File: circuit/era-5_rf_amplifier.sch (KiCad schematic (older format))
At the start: 9 parts, among them J1 CONN_01X04, J2 CONN_01X04, U1 ERA-5+

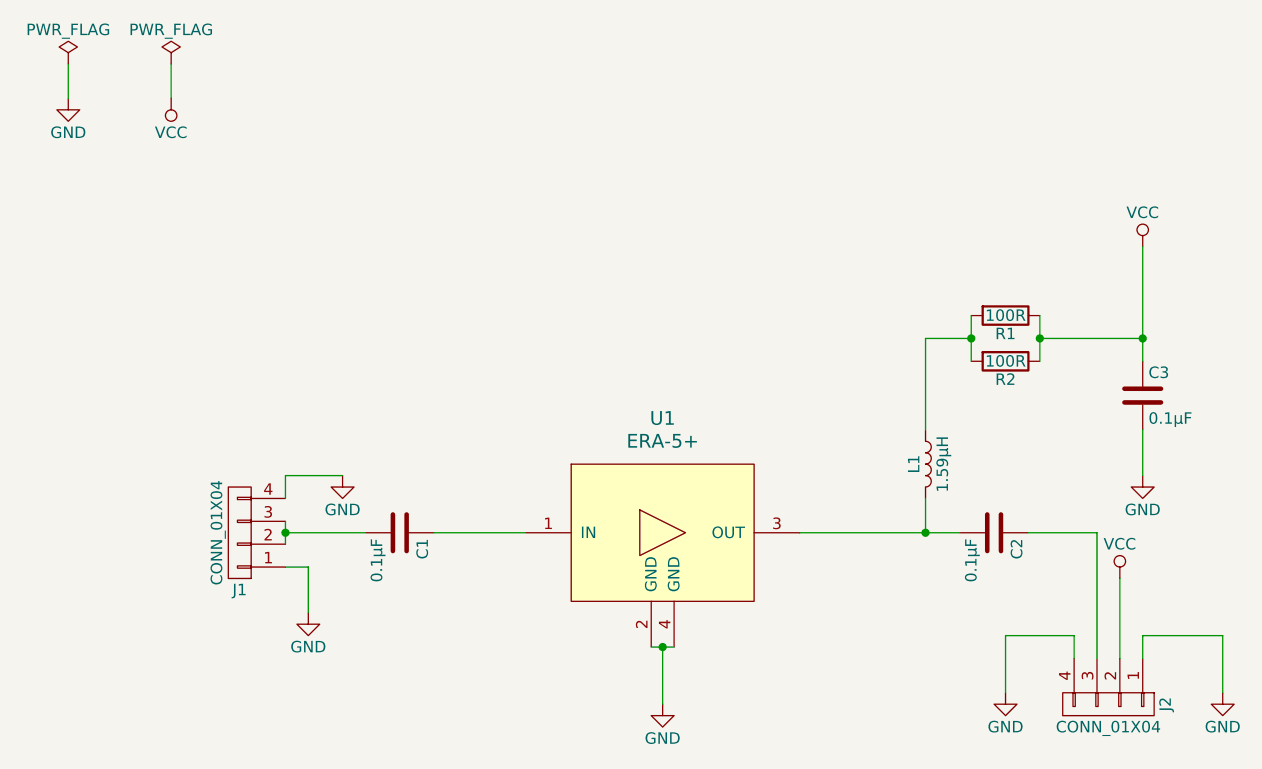
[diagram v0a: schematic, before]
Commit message: rearranged schematics
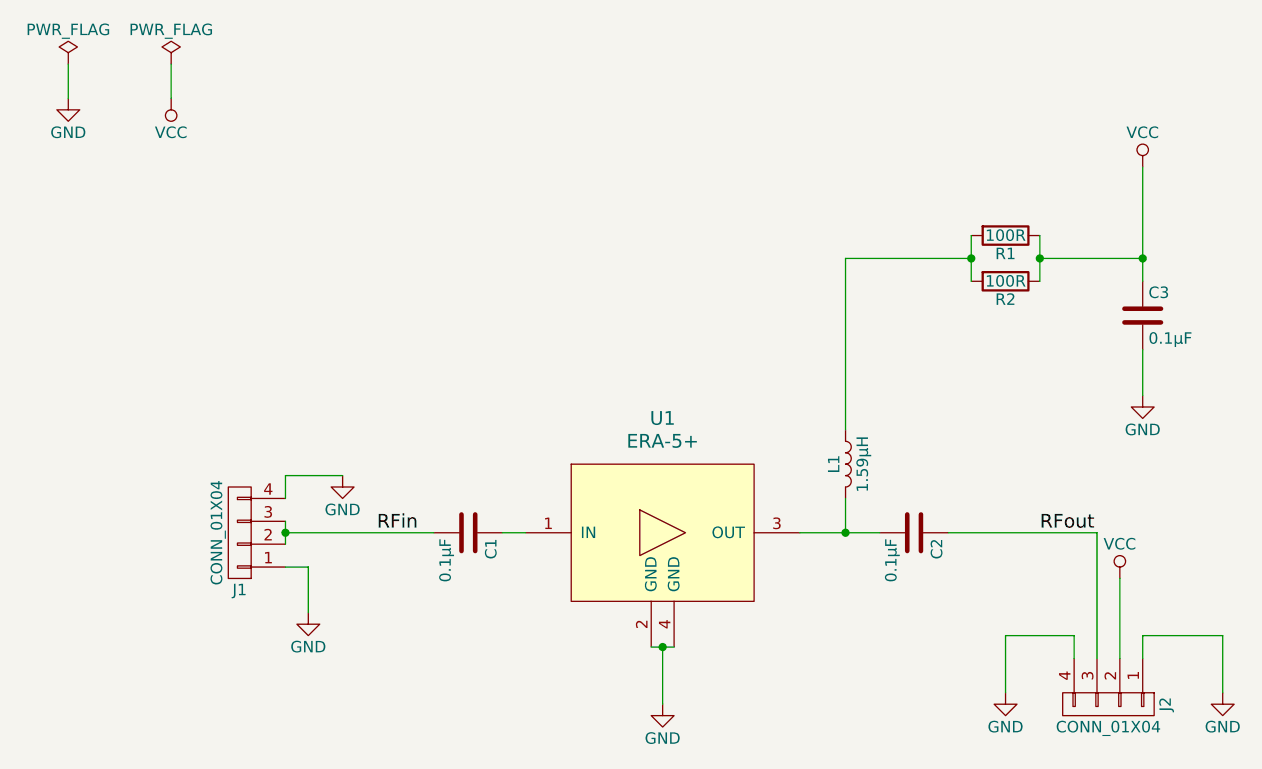
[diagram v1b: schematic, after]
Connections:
- net RFin: now reaches C1.2, J1.2 (P2), J1.3 (P3)
- net RFout: now reaches C2.1, J2.3 (P3)
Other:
- moved on the sheet: C1, C2, C3, L1, R1, R2
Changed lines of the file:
@@
 L C C1
 U 1 1 5931B134
-P 2550 2800
-F 0 "C1" H 2575 2900 50  0000 L CNN
-F 1 "0.1µF" H 2575 2700 50  0000 L CNN
-F 2 "" H 2588 2650 50  0001 C CNN
-F 3 "" H 2550 2800 50  0001 C CNN
-	1    2550 2800
+P 2850 2800
+F 0 "C1" H 2875 2900 50  0000 L CNN
+F 1 "0.1µF" H 2875 2700 50  0000 L CNN
+F 2 "" H 2888 2650 50  0001 C CNN
+F 3 "" H 2850 2800 50  0001 C CNN
+	1    2850 2800
 	0    1    1    0
 $EndComp
@@
 L C C2
 U 1 1 5931B1E4
-P 5150 2800
-F 0 "C2" H 5175 2900 50  0000 L CNN
-F 1 "0.1µF" H 5175 2700 50  0000 L CNN
-F 2 "" H 5188 2650 50  0001 C CNN
-F 3 "" H 5150 2800 50  0001 C CNN
-	1    5150 2800
+P 4800 2800
+F 0 "C2" H 4825 2900 50  0000 L CNN
+F 1 "0.1µF" H 4825 2700 50  0000 L CNN
+F 2 "" H 4838 2650 50  0001 C CNN
+F 3 "" H 4800 2800 50  0001 C CNN
+	1    4800 2800
 	0    1    1    0
 $EndComp
@@
 L L L1
 U 1 1 5931B2E5
-P 4850 2500
-F 0 "L1" V 4800 2500 50  0000 C CNN
-F 1 "1.59µH" V 4925 2500 50  0000 C CNN
-F 2 "" H 4850 2500 50  0001 C CNN
-F 3 "" H 4850 2500 50  0001 C CNN
-	1    4850 2500
+P 4500 2500
+F 0 "L1" V 4450 2500 50  0000 C CNN
+F 1 "1.59µH" V 4575 2500 50  0000 C CNN
+F 2 "" H 4500 2500 50  0001 C CNN
+F 3 "" H 4500 2500 50  0001 C CNN
+	1    4500 2500
 	1    0    0    -1
 $EndComp
@@
 L R R2
 U 1 1 5931B3DD
-P 5200 2050
-F 0 "R2" V 5280 2050 50  0000 C CNN
-F 1 "100R" V 5200 2050 50  0000 C CNN
-F 2 "" V 5130 2050 50  0001 C CNN
-F 3 "" H 5200 2050 50  0001 C CNN
-	1    5200 2050
+P 5200 1700
+F 0 "R2" V 5280 1700 50  0000 C CNN
+F 1 "100R" V 5200 1700 50  0000 C CNN
+F 2 "" V 5130 1700 50  0001 C CNN
+F 3 "" H 5200 1700 50  0001 C CNN
+	1    5200 1700
 	0    1    1    0
 $EndComp
@@
 L R R1
 U 1 1 5931B444
-P 5200 1850
-F 0 "R1" V 5280 1850 50  0000 C CNN
-F 1 "100R" V 5200 1850 50  0000 C CNN
-F 2 "" V 5130 1850 50  0001 C CNN
-F 3 "" H 5200 1850 50  0001 C CNN
-	1    5200 1850
+P 5200 1500
+F 0 "R1" V 5280 1500 50  0000 C CNN
+F 1 "100R" V 5200 1500 50  0000 C CNN
+F 2 "" V 5130 1500 50  0001 C CNN
+F 3 "" H 5200 1500 50  0001 C CNN
+	1    5200 1500
 	0    1    1    0
 $EndComp
@@
 L C C3
 U 1 1 5931B556
+P 5800 1850
+F 0 "C3" H 5825 1950 50  0000 L CNN
+F 1 "0.1µF" H 5825 1750 50  0000 L CNN
+F 2 "" H 5838 1700 50  0001 C CNN
+F 3 "" H 5800 1850 50  0001 C CNN
+	1    5800 1850
+	1    0    0    -1
+$EndComp
+$Comp
+L GND #PWR01
+U 1 1 5931B719
 P 5800 2200
-F 0 "C3" H 5825 2300 50  0000 L CNN
-F 1 "0.1µF" H 5825 2100 50  0000 L CNN
-F 2 "" H 5838 2050 50  0001 C CNN
+F 0 "#PWR01" H 5800 1950 50  0001 C CNN
+F 1 "GND" H 5800 2050 50  0000 C CNN
+F 2 "" H 5800 2200 50  0001 C CNN
 F 3 "" H 5800 2200 50  0001 C CNN
 	1    5800 2200
@@
 $EndComp
 $Comp
-L GND #PWR01
-U 1 1 5931B719
-P 5800 2550
-F 0 "#PWR01" H 5800 2300 50  0001 C CNN
-F 1 "GND" H 5800 2400 50  0000 C CNN
-F 2 "" H 5800 2550 50  0001 C CNN
-F 3 "" H 5800 2550 50  0001 C CNN
-	1    5800 2550
-	1    0    0    -1
-$EndComp
-$Comp
 L VCC #PWR02
 U 1 1 5931B73F
-P 5800 1550
-F 0 "#PWR02" H 5800 1400 50  0001 C CNN
-F 1 "VCC" H 5800 1700 50  0000 C CNN
-F 2 "" H 5800 1550 50  0001 C CNN
-F 3 "" H 5800 1550 50  0001 C CNN
-	1    5800 1550
-	1    0    0    -1
-$EndComp
-Wire Wire Line
-	5800 2350 5800 2550
-Wire Wire Line
-	5800 1550 5800 2050
-Wire Wire Line
-	5350 1850 5350 2050
-Wire Wire Line
-	5350 1950 5800 1950
-Connection ~ 5800 1950
-Connection ~ 5350 1950
-Wire Wire Line
-	5050 1850 5050 2050
-Wire Wire Line
-	4850 2350 4850 1950
-Wire Wire Line
-	4850 1950 5050 1950
-Connection ~ 5050 1950
-Wire Wire Line
-	4850 2650 4850 2800
-Wire Wire Line
-	4300 2800 5000 2800
+P 5800 1200
+F 0 "#PWR02" H 5800 1050 50  0001 C CNN
+F 1 "VCC" H 5800 1350 50  0000 C CNN
+F 2 "" H 5800 1200 50  0001 C CNN
+F 3 "" H 5800 1200 50  0001 C CNN
+	1    5800 1200
+	1    0    0    -1
+$EndComp
+Wire Wire Line
+	5800 2000 5800 2200
+Wire Wire Line
+	5800 1200 5800 1700
+Wire Wire Line
+	5350 1500 5350 1700
+Wire Wire Line
+	5350 1600 5800 1600
+Connection ~ 5800 1600
+Connection ~ 5350 1600
+Wire Wire Line
+	5050 1500 5050 1700
+Wire Wire Line
+	4500 1600 5050 1600
+Connection ~ 5050 1600
 $Comp
 L CONN_01X04 J1
@@
 	2050 2750 2050 2850
 Wire Wire Line
-	2050 2800 2400 2800
+	2050 2800 2700 2800
 Connection ~ 2050 2800
 $Comp
@@
 	2150 2950 2150 3150
 Wire Wire Line
-	5300 2800 5600 2800
+	4950 2800 5600 2800
 Wire Wire Line
 	5600 2800 5600 3350
@@
 Wire Wire Line
 	5200 3250 5200 3500
-Connection ~ 4850 2800
-Wire Wire Line
-	2700 2800 3100 2800
 $Comp
 L ERA-5+ U1
@@
 Wire Wire Line
 	1100 750  1100 900
+Text Label 5350 2800 0    60   ~ 0
+RFout
+Wire Wire Line
+	3000 2800 3100 2800
+Text Label 2450 2800 0    60   ~ 0
+RFin
+Wire Wire Line
+	4650 2800 4300 2800
+Wire Wire Line
+	4500 2650 4500 2800
+Connection ~ 4500 2800
+Wire Wire Line
+	4500 1600 4500 2350
 $EndSCHEMATC

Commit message: added some footprints
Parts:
- C1, C2, C3: footprint (none) -> Capacitors_SMD:C_1210_HandSoldering
- R1, R2: footprint (none) -> Resistors_SMD:R_1210_HandSoldering
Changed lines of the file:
@@
 LIBS:mc-amplifiers
 LIBS:rfcom
+LIBS:mc-chokes
 LIBS:era-5_rf_amplifier-cache
 EELAYER 25 0
@@
 F 0 "C1" H 2875 2900 50  0000 L CNN
 F 1 "0.1µF" H 2875 2700 50  0000 L CNN
-F 2 "" H 2888 2650 50  0001 C CNN
+F 2 "Capacitors_SMD:C_1210_HandSoldering" H 2888 2650 50  0001 C CNN
 F 3 "" H 2850 2800 50  0001 C CNN
 	1    2850 2800
@@
 F 0 "C2" H 4825 2900 50  0000 L CNN
 F 1 "0.1µF" H 4825 2700 50  0000 L CNN
-F 2 "" H 4838 2650 50  0001 C CNN
+F 2 "Capacitors_SMD:C_1210_HandSoldering" H 4838 2650 50  0001 C CNN
 F 3 "" H 4800 2800 50  0001 C CNN
 	1    4800 2800
@@
 F 0 "R2" V 5280 1700 50  0000 C CNN
 F 1 "100R" V 5200 1700 50  0000 C CNN
-F 2 "" V 5130 1700 50  0001 C CNN
+F 2 "Resistors_SMD:R_1210_HandSoldering" V 5130 1700 50  0001 C CNN
 F 3 "" H 5200 1700 50  0001 C CNN
 	1    5200 1700
@@
 F 0 "R1" V 5280 1500 50  0000 C CNN
 F 1 "100R" V 5200 1500 50  0000 C CNN
-F 2 "" V 5130 1500 50  0001 C CNN
+F 2 "Resistors_SMD:R_1210_HandSoldering" V 5130 1500 50  0001 C CNN
 F 3 "" H 5200 1500 50  0001 C CNN
 	1    5200 1500
@@
 F 0 "C3" H 5825 1950 50  0000 L CNN
 F 1 "0.1µF" H 5825 1750 50  0000 L CNN
-F 2 "" H 5838 1700 50  0001 C CNN
+F 2 "Capacitors_SMD:C_1210_HandSoldering" H 5838 1700 50  0001 C CNN
 F 3 "" H 5800 1850 50  0001 C CNN
 	1    5800 1850
